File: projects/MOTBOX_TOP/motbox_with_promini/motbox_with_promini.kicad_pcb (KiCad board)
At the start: 2 copper layers, 90 x 71.2 mm, 27 parts, among them J1 12V IN, J2 Manual EN, J3 OBS_IR_TX, J4 OP_CL_OBS_DET_LED, J5 OBS IR RX, J6 Open Close Done, J7 Motor, P1 Digital, P2 ADC, P3 COM, P4 ADC, P5 Analog, U1 LM2575-5.0BU, U2 LM393, U3 L293D

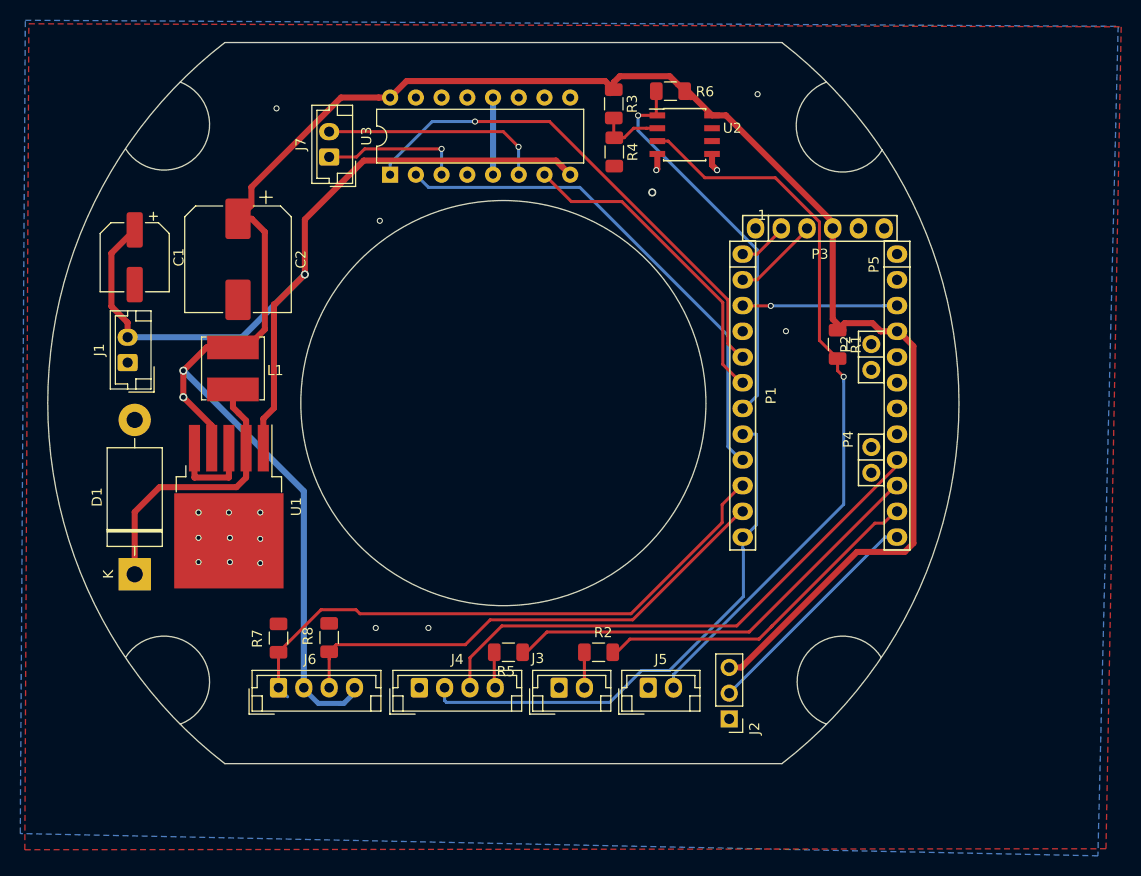
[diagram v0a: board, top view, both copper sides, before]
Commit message: Seems to be final version with promini
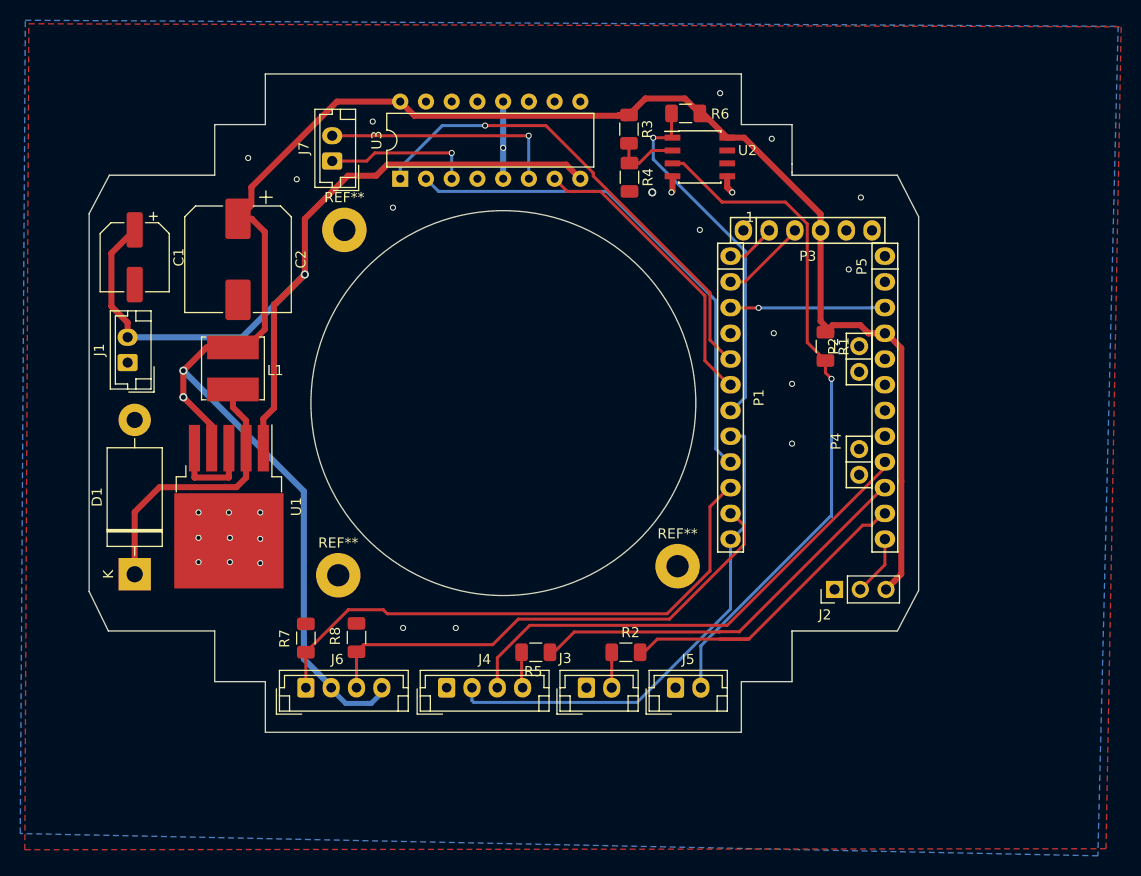
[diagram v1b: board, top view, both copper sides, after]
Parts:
- added REF**: MountingHole_2.2mm_M2_Pad, MountingHole:MountingHole_2.2mm_M2_Pad, F.Cu at (99.6, 39.0)
- added REF**: MountingHole_2.2mm_M2_Pad, MountingHole:MountingHole_2.2mm_M2_Pad, F.Cu at (99.0, 73.1)
- added REF**: MountingHole_2.2mm_M2_Pad, MountingHole:MountingHole_2.2mm_M2_Pad, F.Cu at (132.5, 72.2)
- moved J2 16.5 mm to (148.0, 74.5), turned to 90 degrees
- moved R3 2.92 mm to (127.7, 29.1)
- moved R4 2.92 mm to (127.8, 33.8)
- moved J5 2.70 mm to (132.3, 84.2)
- moved J3 2.70 mm to (123.5, 84.2)
- moved J4 2.70 mm to (109.7, 84.2)
- moved J6 2.70 mm to (95.8, 84.2)
- moved R2 2.70 mm to (127.4, 80.7)
- moved R5 2.70 mm to (118.5, 80.7)
- moved R7 2.70 mm to (95.8, 79.3)
- moved R8 2.70 mm to (100.8, 79.2)
- moved U2 2.66 mm to (134.7, 31.8)
- moved R6 2.66 mm to (133.3, 27.5)
- moved P1 1.22 mm to (137.7, 41.6)
- moved R1 1.22 mm to (147.1, 50.5)
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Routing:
- net +5V: track 216.8 -> 198.0 mm
- net /10: track 23.1 -> 6.29 mm
- net Net-(J5-Pad2): track 73.9 -> 68.9 mm
- net /13: track 53.5 -> 49.6 mm
- net /12: track 43.8 -> 39.9 mm
- net /5: track 53.5 -> 50.0 mm
- net /4: track 39.3 -> 36.2 mm
- net /7: track 58.8 -> 56.2 mm
- net /3: track 31.7 -> 29.6 mm
- net /2: track 49.8 -> 47.9 mm
- net Net-(J7-Pad2): track 22.1 -> 23.7 mm
- net /11: track 34.0 -> 32.6 mm
- net +12V: track 88.2 -> 89.1 mm
- net Net-(J7-Pad1): track 14.0 -> 14.7 mm
- net GND: vias 18 -> 27
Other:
- board size 90 x 71.2 mm -> 81.9 x 65 mm
